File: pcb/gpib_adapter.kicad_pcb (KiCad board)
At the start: 2 copper layers, 73 x 41 mm, 36 parts, among them CON1 AVR-ISP-6, P2 USB, P3 GPIO, P5 GPIB, U1 SN75160, U2 SN75161, U3 FT230XQ, U4 AT90CAN128-A

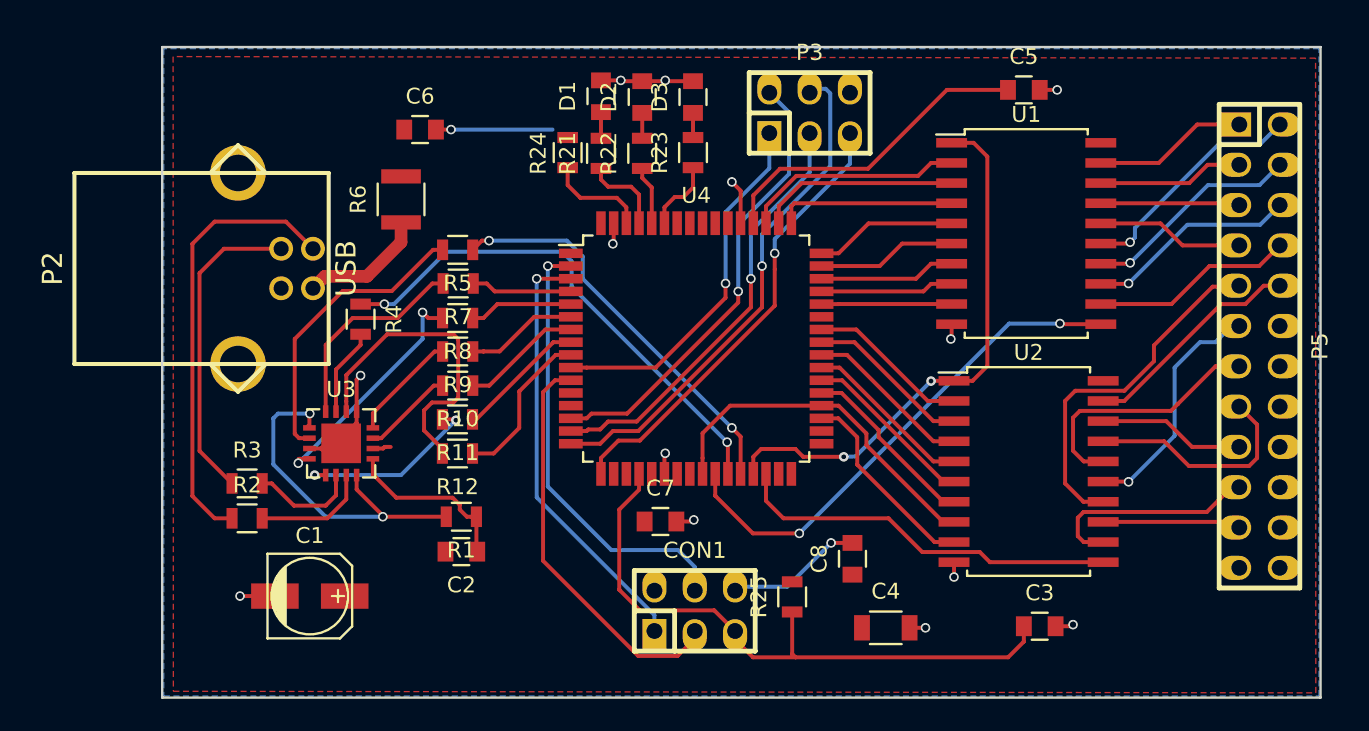
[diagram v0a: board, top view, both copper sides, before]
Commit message: updating hardware
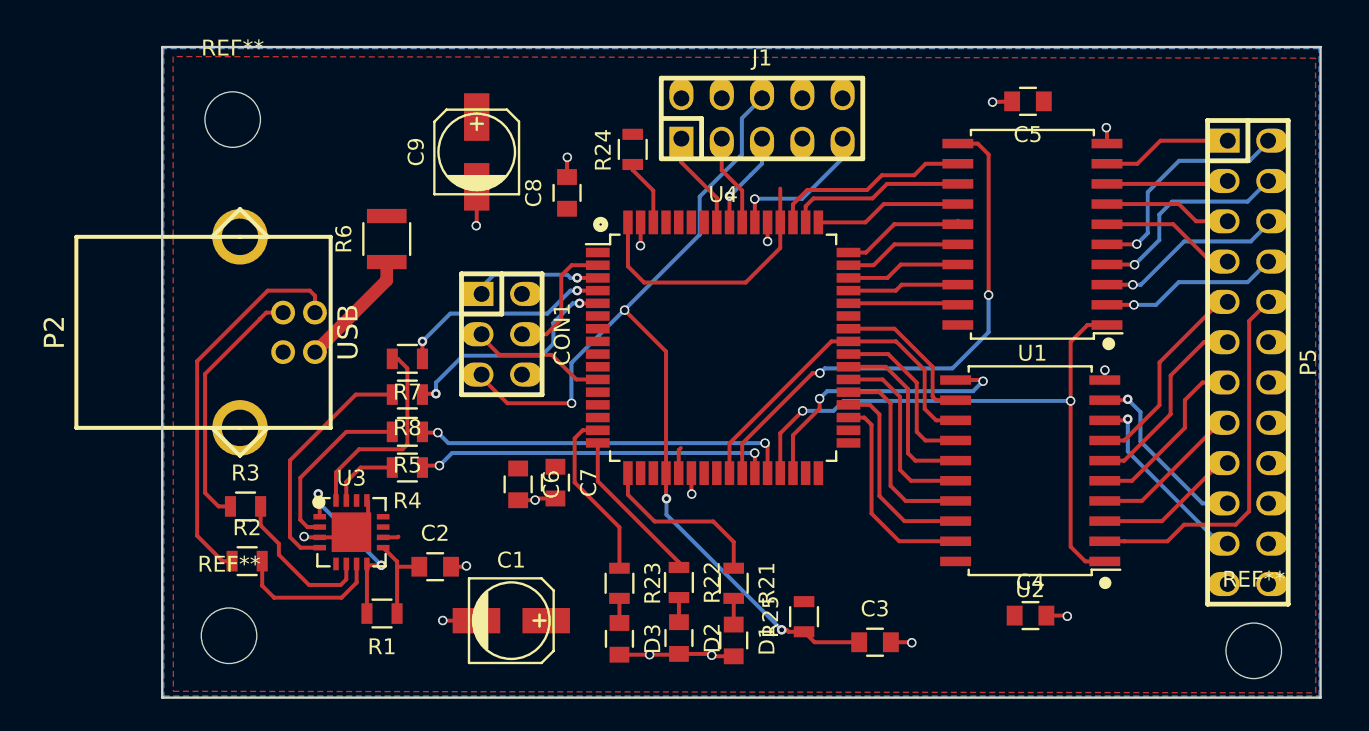
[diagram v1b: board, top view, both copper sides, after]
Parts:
- removed P3: GPIO, w_pin_strip:pin_socket_3x2
- removed R10, R11, R12, R9: R, Resistors_SMD:R_0805
- added C9: 22µ, Capacitors_SMD:c_elec_5x5.3, F.Cu at (131.2, 80.8)
- added J1: HEADER_5x2, w_pin_strip:pin_strip_5x2, F.Cu at (149.2, 78.7)
- added REF**: MountingHole_3-5mm, Mounting_Holes:MountingHole_3-5mm, F.Cu at (115.8, 78.8)
- added REF**: MountingHole_3-5mm, Mounting_Holes:MountingHole_3-5mm, F.Cu at (115.6, 111.3)
- added REF**: MountingHole_3-5mm, Mounting_Holes:MountingHole_3-5mm, F.Cu at (180.2, 112.2)
- C4: footprint Capacitors_SMD:C_1206 -> Capacitors_SMD:C_0805
- moved D1 35.3 mm to (147.4, 111.6), turned to 270 degrees
- moved D3 34.5 mm to (140.2, 111.5), turned to 270 degrees
- moved D2 34.2 mm to (144.0, 111.4), turned to 270 degrees
- moved C8 29.2 mm to (136.9, 83.4)
- moved R21 28.4 mm to (147.4, 108.0), turned to 270 degrees
- moved R23 27.5 mm to (140.2, 108.0), turned to 270 degrees
- moved R22 27.1 mm to (144.0, 107.9), turned to 270 degrees
- moved C6 23.2 mm to (133.8, 101.8), turned to 270 degrees
- moved CON1 21.3 mm to (132.8, 92.3), turned to 270 degrees
- moved C1 12.8 mm to (133.4, 110.3)
- moved R5 11.9 mm to (126.8, 98.5)
- moved C3 10.4 mm to (156.3, 111.7)
- moved R4 9.80 mm to (126.8, 100.7), turned to 180 degrees
- moved C4 9.15 mm to (166.1, 110.0)
- moved R1 7.89 mm to (125.2, 109.9)
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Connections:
- R21 pad 1: Net-(R21-Pad1) -> /TALK
- R22 pad 1: Net-(R22-Pad1) -> /MODE
- R23 pad 1: Net-(R23-Pad1) -> /PWR
- U1 pad 12: /DIO8 B -> /DIO1
- U1 pad 13: /DIO7 B -> /DIO2
- U1 pad 14: /DIO6 B -> /DIO3
- U1 pad 15: /DIO5 B -> /DIO4
- U1 pad 16: /DIO4 B -> /DIO5
- U1 pad 17: /DIO3 B -> /DIO6
- U1 pad 18: /DIO2 B -> /DIO7
- U1 pad 19: /DIO1 B -> /DIO8
- U1 pad 2: /DIO1 -> /DIO8 B
- U1 pad 3: /DIO2 -> /DIO7 B
- U1 pad 4: /DIO3 -> /DIO6 B
- U1 pad 5: /DIO4 -> /DIO5 B
- U1 pad 6: /DIO5 -> /DIO4 B
- U1 pad 7: /DIO6 -> /DIO3 B
- U1 pad 8: /DIO7 -> /DIO2 B
- U1 pad 9: /DIO8 -> /DIO1 B
- U2 pad 12: /SRQ B -> /SRQ
- U2 pad 13: /ATN B -> /ATN
- U2 pad 14: /EOI B -> /EOI
- U2 pad 15: /DAV B -> /DAV
- U2 pad 16: /NRFD B -> /NRFD
- U2 pad 17: /NDAC B -> /NDAC
- U2 pad 18: /IFC B -> /IFC
- U2 pad 19: /REN B -> /REN
- U2 pad 2: /REN -> /REN B
- U2 pad 3: /IFC -> /IFC B
- U2 pad 4: /NDAC -> /NDAC B
- U2 pad 5: /NRFD -> /NRFD B
- U2 pad 6: /DAV -> /DAV B
- U2 pad 7: /EOI -> /EOI B
- U2 pad 8: /ATN -> /ATN B
- U2 pad 9: /SRQ -> /SRQ B
- U3 pad 11: Net-(R10-Pad2) -> (no net)
- U3 pad 12: Net-(R9-Pad2) -> (no net)
- U3 pad 14: Net-(R12-Pad2) -> (no net)
- U3 pad 5: Net-(R11-Pad2) -> (no net)
- U4 pad 10: /GPIO1 -> (no net)
- U4 pad 14: /GPIO2 -> (no net)
- U4 pad 15: /GPIO3 -> /PWR
- U4 pad 16: /GPIO4 -> /MODE
- U4 pad 17: /GPIO5 -> /TALK
- U4 pad 35: /SRQ -> /REN
- U4 pad 36: /ATN -> /IFC
- U4 pad 37: /EOI -> /NDAC
- U4 pad 38: /DAV -> /NRFD
- U4 pad 39: /NRFD -> /DAV
- U4 pad 40: /NDAC -> /EOI
- U4 pad 41: /IFC -> /ATN
- U4 pad 42: /REN -> /SRQ
- U4 pad 54: (no net) -> /TDI
- U4 pad 55: (no net) -> /TDO
- U4 pad 56: (no net) -> /TMS
- U4 pad 57: (no net) -> /TCK
- U4 pad 59: Net-(R23-Pad1) -> (no net)
- U4 pad 6: Net-(R9-Pad1) -> (no net)
- U4 pad 60: Net-(R22-Pad1) -> (no net)
- U4 pad 61: Net-(R21-Pad1) -> (no net)
- U4 pad 7: Net-(R10-Pad1) -> (no net)
- U4 pad 8: Net-(R11-Pad1) -> (no net)
- U4 pad 9: Net-(R12-Pad1) -> (no net)
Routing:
- net /GPIO4: track 32.3 -> 0.00 mm, vias 1 -> 0
- net /GPIO2: track 28.9 -> 0.00 mm, vias 1 -> 0
- net /GPIO5: track 28.5 -> 0.00 mm, vias 1 -> 0
- net /GPIO3: track 26.8 -> 0.00 mm, vias 1 -> 0
- net /GPIO1: track 22.8 -> 0.00 mm, vias 1 -> 0
- net /RESET: track 40.0 -> 60.5 mm, vias 0 -> 4
- net Net-(R12-Pad2): track 19.9 -> 0.00 mm
- net /MOSI: track 28.0 -> 8.19 mm, vias 1 -> 0
- net /MISO: track 27.9 -> 8.55 mm
- net /SCK: track 25.4 -> 8.93 mm
- net GND: track 49.4 -> 34.1 mm, vias 15 -> 16
- net Net-(R11-Pad2): track 11.9 -> 0.00 mm, vias 2 -> 0
- net /PWR: track 0.00 -> 11.0 mm
- net /TALK: track 0.00 -> 10.9 mm
- net /EOI B: track 23.7 -> 12.9 mm
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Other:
- board text added: "GPIB-USB Converter V1.1 14.10.2015"
- board text removed: "GPIB-USB Converter V1.1 10.10.2015"
